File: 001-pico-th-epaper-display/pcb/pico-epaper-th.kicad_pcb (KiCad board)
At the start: 2 copper layers, 70 x 70 mm, 17 parts, among them Q1 AO3407, U1 GY-SHT31-D, U2 TPL5110, U3 WS_1_54_epaper_module

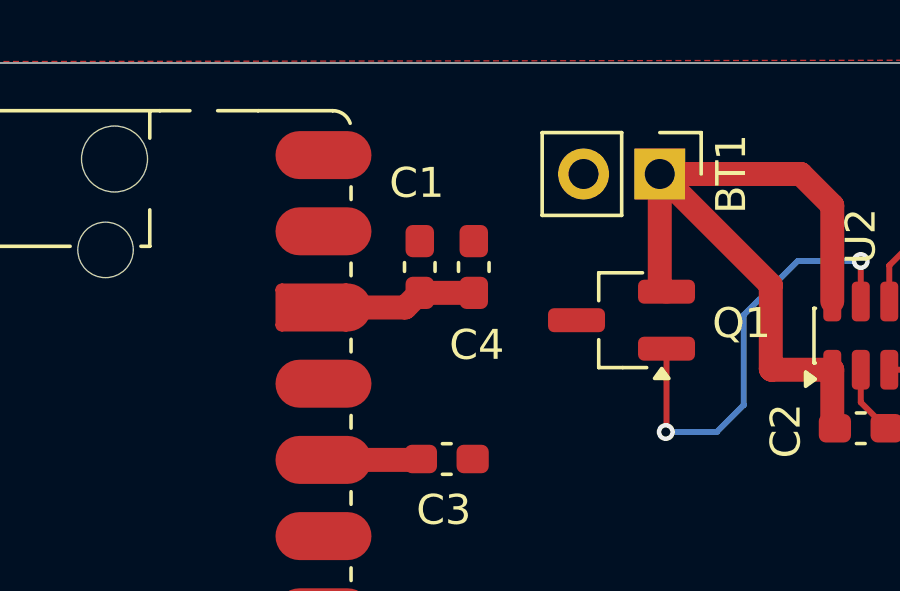
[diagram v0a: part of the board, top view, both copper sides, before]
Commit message: pcb rounting
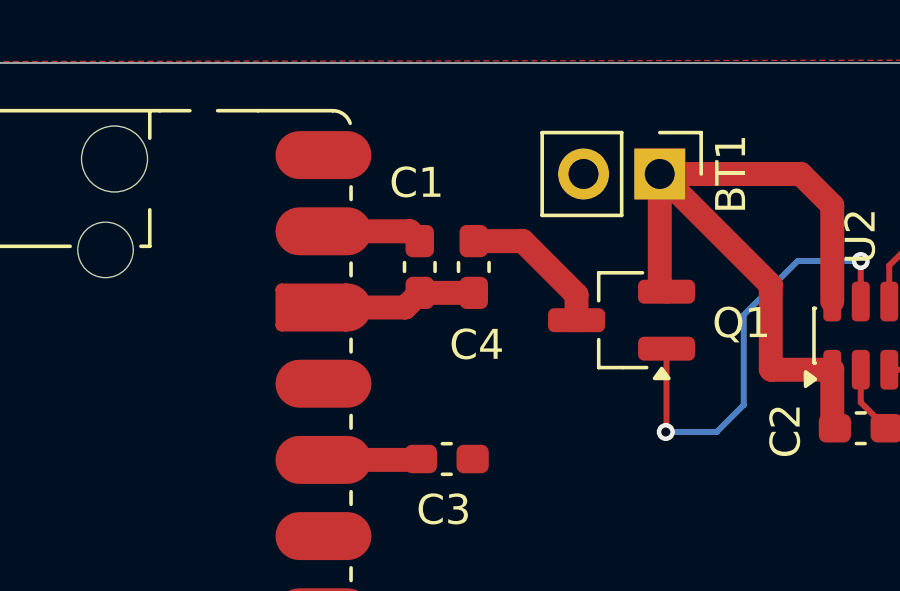
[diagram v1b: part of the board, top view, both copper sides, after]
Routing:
- net Net-(A1-VSYS): track 0.00 -> 8.36 mm
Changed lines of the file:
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@@
+	)
+	(segment
+		(start 147.9725 77.91)
+		(end 148.3 78.2375)
+		(width 0.8)
+		(layer "F.Cu")
+		(net "Net-(A1-VSYS)")
+	)
+	(segment
+		(start 145.09 77.91)
+		(end 147.9725 77.91)
+		(width 0.8)
+		(layer "F.Cu")
+		(net "Net-(A1-VSYS)")
+	)
+	(segment
+		(start 151.7375 78.2375)
+		(end 153.525 80.025)
+		(width 0.8)
+		(layer "F.Cu")
+		(net "Net-(A1-VSYS)")
+	)
+	(segment
+		(start 153.525 80.025)
+		(end 153.525 80.873089)
+		(width 0.8)
+		(layer "F.Cu")
+		(net "Net-(A1-VSYS)")
+	)
+	(segment
+		(start 150.1 78.2375)
+		(end 151.7375 78.2375)
+		(width 0.8)
+		(layer "F.Cu")
+		(net "Net-(A1-VSYS)")
 	)
 	(segment
